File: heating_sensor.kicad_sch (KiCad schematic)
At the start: 3 parts

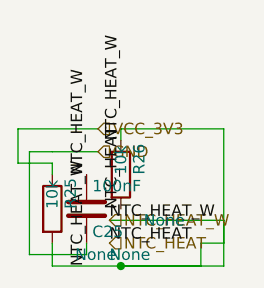
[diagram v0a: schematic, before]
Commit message: all unit test pass
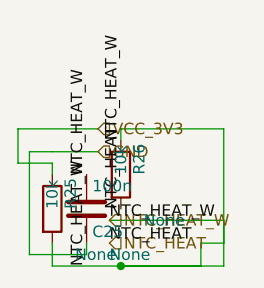
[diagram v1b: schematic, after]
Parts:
- C25: value 100nF -> 100n
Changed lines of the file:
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@@
 			)
 		)
-		(property "Value" "100nF"
+		(property "Value" "100n"
 			(at 18.415 15.24 0.0000)
 			(effects
@@
 		(instances
 			(project "Untitled"
-				(path "/2b46367b-7f7a-4d0b-a981-14ef6f17f746"
+				(path "/ce240599-ae42-4376-828a-09a891a5e9c6"
 					(reference "C25")
 					(unit 1)
@@
 		(instances
 			(project "Untitled"
-				(path "/2b46367b-7f7a-4d0b-a981-14ef6f17f746"
+				(path "/ce240599-ae42-4376-828a-09a891a5e9c6"
 					(reference "R25")
 					(unit 1)
@@
 		(instances
 			(project "Untitled"
-				(path "/2b46367b-7f7a-4d0b-a981-14ef6f17f746"
+				(path "/ce240599-ae42-4376-828a-09a891a5e9c6"
 					(reference "R26")
 					(unit 1)
